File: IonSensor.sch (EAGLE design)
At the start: 43 parts, among them IC1 QUAD_OPAMPD, IC2 QUAD_OPAMPD, IC3 QUAD_OPAMPD

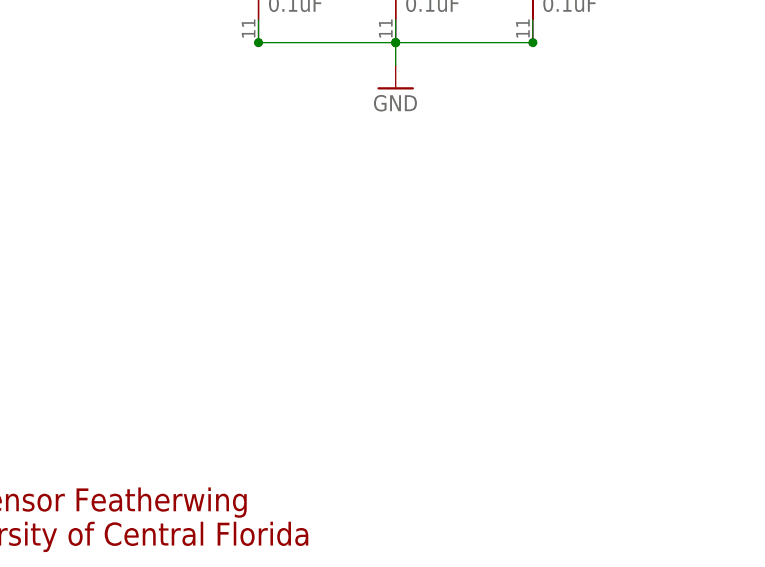
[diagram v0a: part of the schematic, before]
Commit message: Added JST XH Connector
Added JST XH connector. TODO: Wire channels up!
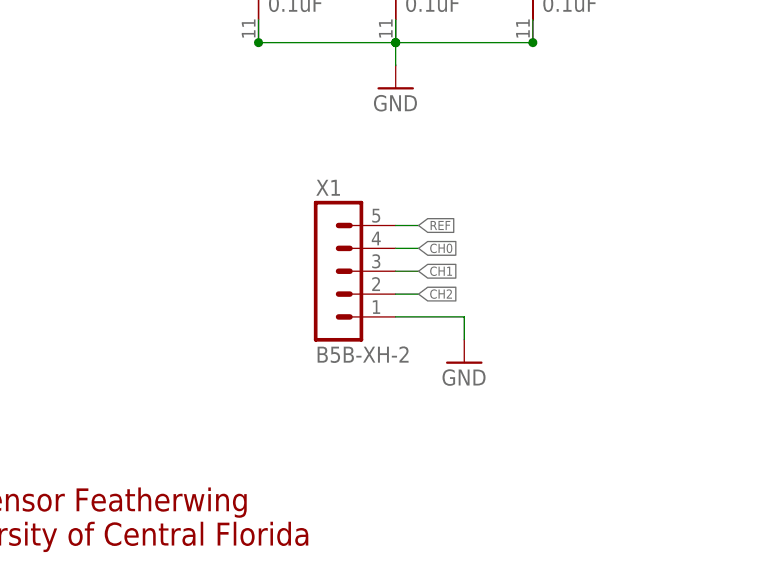
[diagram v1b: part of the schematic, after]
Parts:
- added X1: B5B-XH-2, con-JST XH:B5B-XH-2
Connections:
- net CH0: now also X1.4
- net CH1: now also X1.3
- net CH2: now also X1.2
- net GND: now also X1.1
- net REF: now also X1.5
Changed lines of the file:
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@@
 <part name="GND13" library="supply1" library_urn="urn:adsk.eagle:library:371" deviceset="GND" device=""/>
 <part name="GND14" library="supply1" library_urn="urn:adsk.eagle:library:371" deviceset="GND" device=""/>
+<part name="X1" library="con-JST XH" deviceset="B5B-XH" device="-2"/>
+<part name="GND15" library="supply1" library_urn="urn:adsk.eagle:library:371" deviceset="GND" device=""/>
 </parts>
 <sheets>
@@
 <instance part="GND14" gate="1" x="71.12" y="35.56" smashed="yes">
 <attribute name="VALUE" x="68.58" y="33.02" size="1.778" layer="96"/>
+</instance>
+<instance part="X1" gate="G$1" x="195.58" y="58.42" smashed="yes">
+<attribute name="VALUE" x="194.31" y="48.26" size="1.778" layer="96"/>
+<attribute name="NAME" x="194.31" y="66.802" size="1.778" layer="95"/>
+</instance>
+<instance part="GND15" gate="1" x="210.82" y="48.26" smashed="yes">
+<attribute name="VALUE" x="208.28" y="45.72" size="1.778" layer="96"/>
 </instance>
 </instances>
@@
 <wire x1="12.7" y1="170.18" x2="17.78" y2="170.18" width="0.1524" layer="91"/>
 </segment>
+<segment>
+<pinref part="X1" gate="G$1" pin="4"/>
+<wire x1="205.74" y1="60.96" x2="203.2" y2="60.96" width="0.1524" layer="91"/>
+<label x="205.74" y="60.96" size="1.016" layer="95" xref="yes"/>
+</segment>
 </net>
 <net name="REF" class="0">
@@
 <label x="12.7" y="30.48" size="1.27" layer="95" rot="R180" xref="yes"/>
 </segment>
+<segment>
+<pinref part="X1" gate="G$1" pin="5"/>
+<wire x1="205.74" y1="63.5" x2="203.2" y2="63.5" width="0.1524" layer="91"/>
+<label x="205.74" y="63.5" size="1.016" layer="95" xref="yes"/>
+</segment>
 </net>
 <net name="CH1" class="0">
@@
 <wire x1="12.7" y1="114.3" x2="17.78" y2="114.3" width="0.1524" layer="91"/>
 </segment>
+<segment>
+<pinref part="X1" gate="G$1" pin="3"/>
+<wire x1="205.74" y1="58.42" x2="203.2" y2="58.42" width="0.1524" layer="91"/>
+<label x="205.74" y="58.42" size="1.016" layer="95" xref="yes"/>
+</segment>
 </net>
 <net name="CH2" class="0">
@@
 <wire x1="12.7" y1="58.42" x2="17.78" y2="58.42" width="0.1524" layer="91"/>
 <label x="12.7" y="58.42" size="1.27" layer="95" rot="R180" xref="yes"/>
+</segment>
+<segment>
+<pinref part="X1" gate="G$1" pin="2"/>
+<wire x1="205.74" y1="55.88" x2="203.2" y2="55.88" width="0.1524" layer="91"/>
+<label x="205.74" y="55.88" size="1.016" layer="95" xref="yes"/>
 </segment>
 </net>
@@
 <wire x1="71.12" y1="38.1" x2="73.66" y2="38.1" width="0.1524" layer="91"/>
 </segment>
-</net>
+<segment>
+<pinref part="X1" gate="G$1" pin="1"/>
+<wire x1="210.82" y1="50.8" x2="210.82" y2="53.34" width="0.1524" layer="91"/>
+<wire x1="210.82" y1="53.34" x2="203.2" y2="53.34" width="0.1524" layer="91"/>
+<pinref part="GND15" gate="1" pin="GND"/>
+</segment>
+</net>

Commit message: Revert "Added JST XH Connector"
This reverts commit 28e9dc296f10d82968848f6f33b36970200c6171.
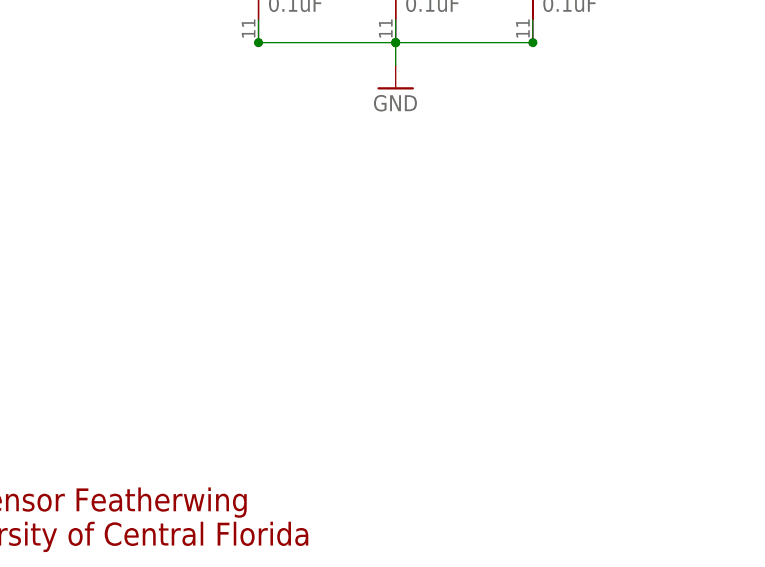
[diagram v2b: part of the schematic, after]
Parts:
- removed X1: B5B-XH-2, con-JST XH:B5B-XH-2
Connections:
- net CH0: no longer X1.4
- net CH1: no longer X1.3
- net CH2: no longer X1.2
- net GND: no longer X1.1
- net REF: no longer X1.5
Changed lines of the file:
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@@
 <part name="GND13" library="supply1" library_urn="urn:adsk.eagle:library:371" deviceset="GND" device=""/>
 <part name="GND14" library="supply1" library_urn="urn:adsk.eagle:library:371" deviceset="GND" device=""/>
-<part name="X1" library="con-JST XH" deviceset="B5B-XH" device="-2"/>
-<part name="GND15" library="supply1" library_urn="urn:adsk.eagle:library:371" deviceset="GND" device=""/>
 </parts>
 <sheets>
@@
 <instance part="GND14" gate="1" x="71.12" y="35.56" smashed="yes">
 <attribute name="VALUE" x="68.58" y="33.02" size="1.778" layer="96"/>
-</instance>
-<instance part="X1" gate="G$1" x="195.58" y="58.42" smashed="yes">
-<attribute name="VALUE" x="194.31" y="48.26" size="1.778" layer="96"/>
-<attribute name="NAME" x="194.31" y="66.802" size="1.778" layer="95"/>
-</instance>
-<instance part="GND15" gate="1" x="210.82" y="48.26" smashed="yes">
-<attribute name="VALUE" x="208.28" y="45.72" size="1.778" layer="96"/>
 </instance>
 </instances>
@@
 <wire x1="12.7" y1="170.18" x2="17.78" y2="170.18" width="0.1524" layer="91"/>
 </segment>
-<segment>
-<pinref part="X1" gate="G$1" pin="4"/>
-<wire x1="205.74" y1="60.96" x2="203.2" y2="60.96" width="0.1524" layer="91"/>
-<label x="205.74" y="60.96" size="1.016" layer="95" xref="yes"/>
-</segment>
 </net>
 <net name="REF" class="0">
@@
 <label x="12.7" y="30.48" size="1.27" layer="95" rot="R180" xref="yes"/>
 </segment>
-<segment>
-<pinref part="X1" gate="G$1" pin="5"/>
-<wire x1="205.74" y1="63.5" x2="203.2" y2="63.5" width="0.1524" layer="91"/>
-<label x="205.74" y="63.5" size="1.016" layer="95" xref="yes"/>
-</segment>
 </net>
 <net name="CH1" class="0">
@@
 <wire x1="12.7" y1="114.3" x2="17.78" y2="114.3" width="0.1524" layer="91"/>
 </segment>
-<segment>
-<pinref part="X1" gate="G$1" pin="3"/>
-<wire x1="205.74" y1="58.42" x2="203.2" y2="58.42" width="0.1524" layer="91"/>
-<label x="205.74" y="58.42" size="1.016" layer="95" xref="yes"/>
-</segment>
 </net>
 <net name="CH2" class="0">
@@
 <wire x1="12.7" y1="58.42" x2="17.78" y2="58.42" width="0.1524" layer="91"/>
 <label x="12.7" y="58.42" size="1.27" layer="95" rot="R180" xref="yes"/>
-</segment>
-<segment>
-<pinref part="X1" gate="G$1" pin="2"/>
-<wire x1="205.74" y1="55.88" x2="203.2" y2="55.88" width="0.1524" layer="91"/>
-<label x="205.74" y="55.88" size="1.016" layer="95" xref="yes"/>
 </segment>
 </net>
@@
 <wire x1="71.12" y1="38.1" x2="73.66" y2="38.1" width="0.1524" layer="91"/>
 </segment>
-<segment>
-<pinref part="X1" gate="G$1" pin="1"/>
-<wire x1="210.82" y1="50.8" x2="210.82" y2="53.34" width="0.1524" layer="91"/>
-<wire x1="210.82" y1="53.34" x2="203.2" y2="53.34" width="0.1524" layer="91"/>
-<pinref part="GND15" gate="1" pin="GND"/>
-</segment>
-</net>
+</net>
